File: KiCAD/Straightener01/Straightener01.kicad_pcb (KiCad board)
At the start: 4 copper layers, 56 x 20 mm, 13 parts, among them IC1 LT3045EDD, J1 C112640, J2 C112640

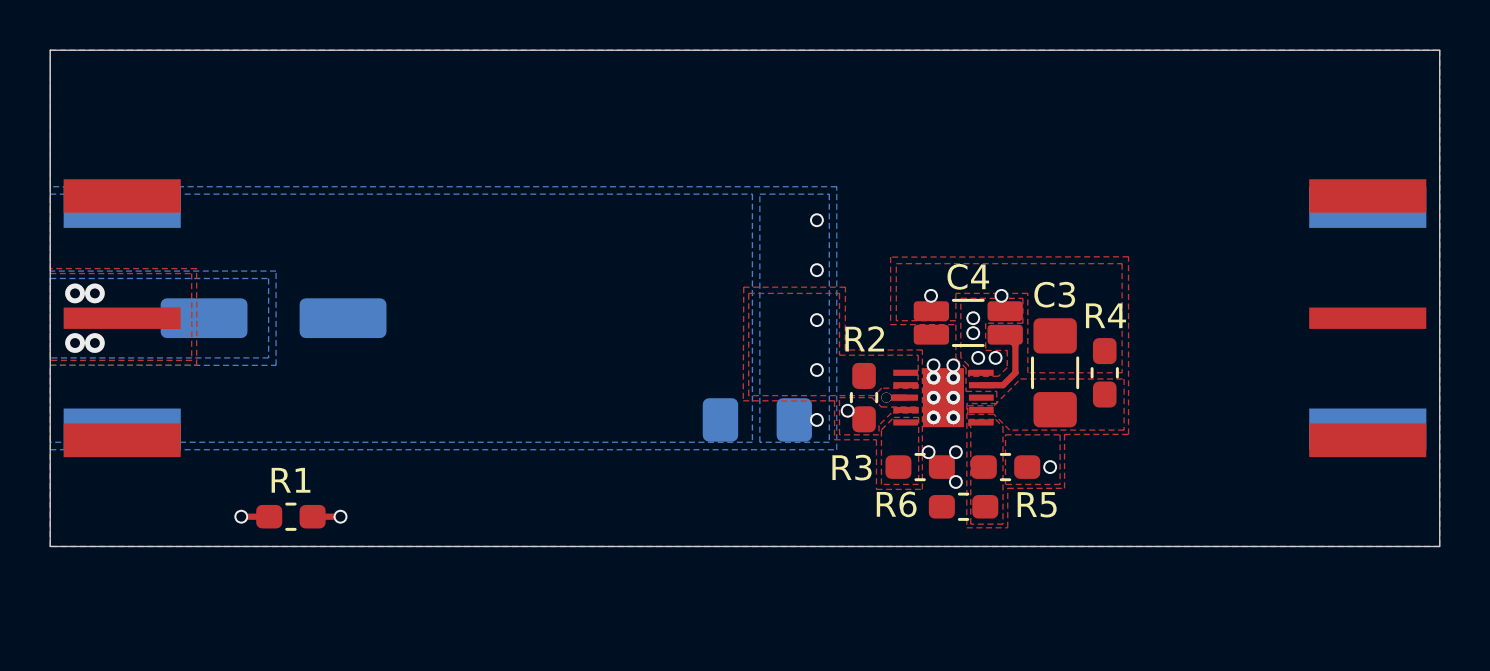
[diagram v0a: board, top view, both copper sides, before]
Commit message: finished up Straightener01
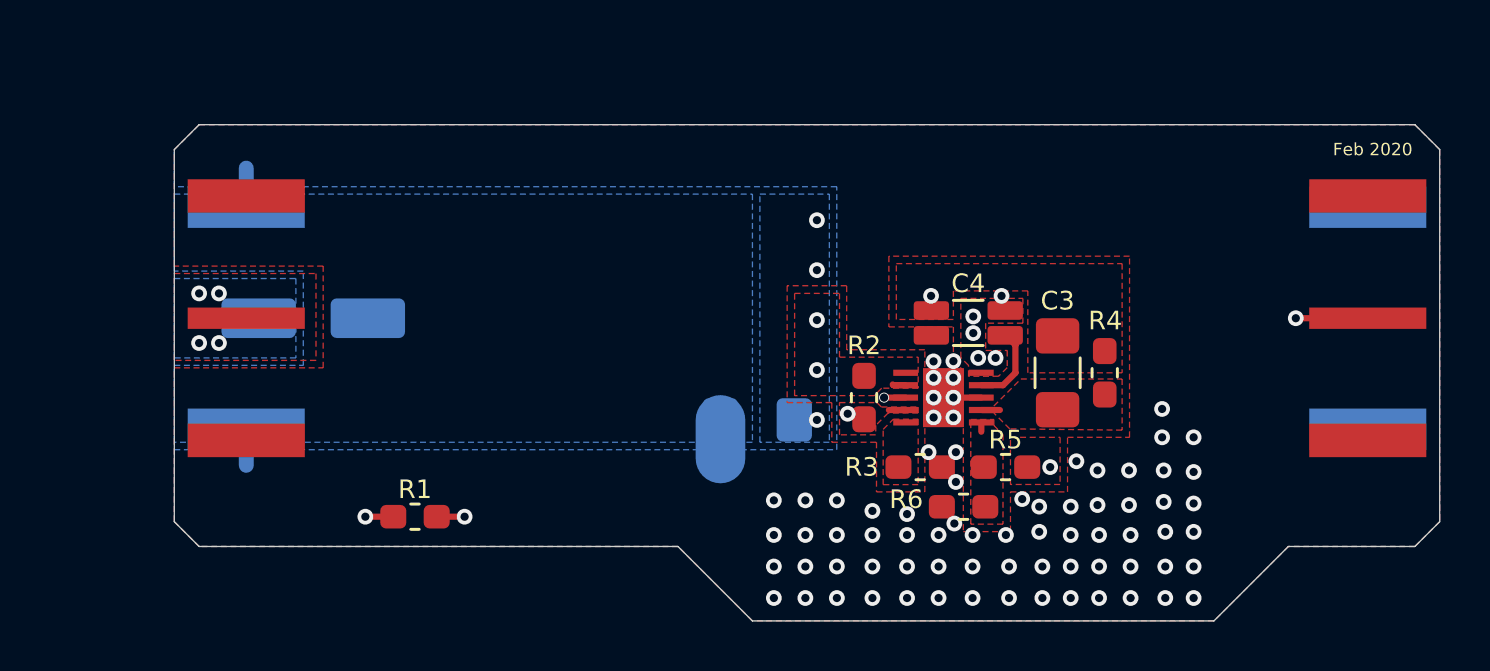
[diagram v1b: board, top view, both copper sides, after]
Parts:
- C1: footprint Capacitor_SMD:CP_Elec_6.3x5.4 -> Capacitor_SMD:CP_Elec_5x5.3
- moved J1 5.00 mm to (104.9, 100.8)
- moved R1 5.00 mm to (111.7, 108.8)
- moved C1 1.60 mm to (107.6, 100.8)
- moved C3 0.10 mm to (137.6, 103.0)
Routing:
- net GND: track 0.00 -> 5.71 mm, vias 11 -> 74
- net /EN_UV: track 27.0 -> 21.5 mm
- net /VOUT: track 6.27 -> 9.17 mm, vias 6 -> 7
- net /SET: track 0.00 -> 0.75 mm
- net /PG: track 0.00 -> 0.67 mm
- net /VIN: track 13.1 -> 13.6 mm
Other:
- board size 56 x 20 mm -> 51 x 20 mm
- board text added: "Dylan Oh"
- board text added: "Feb 2020"
- board text added: "Straightener01"
